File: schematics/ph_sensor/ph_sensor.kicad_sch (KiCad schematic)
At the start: 4 parts, among them U1 MCP3008

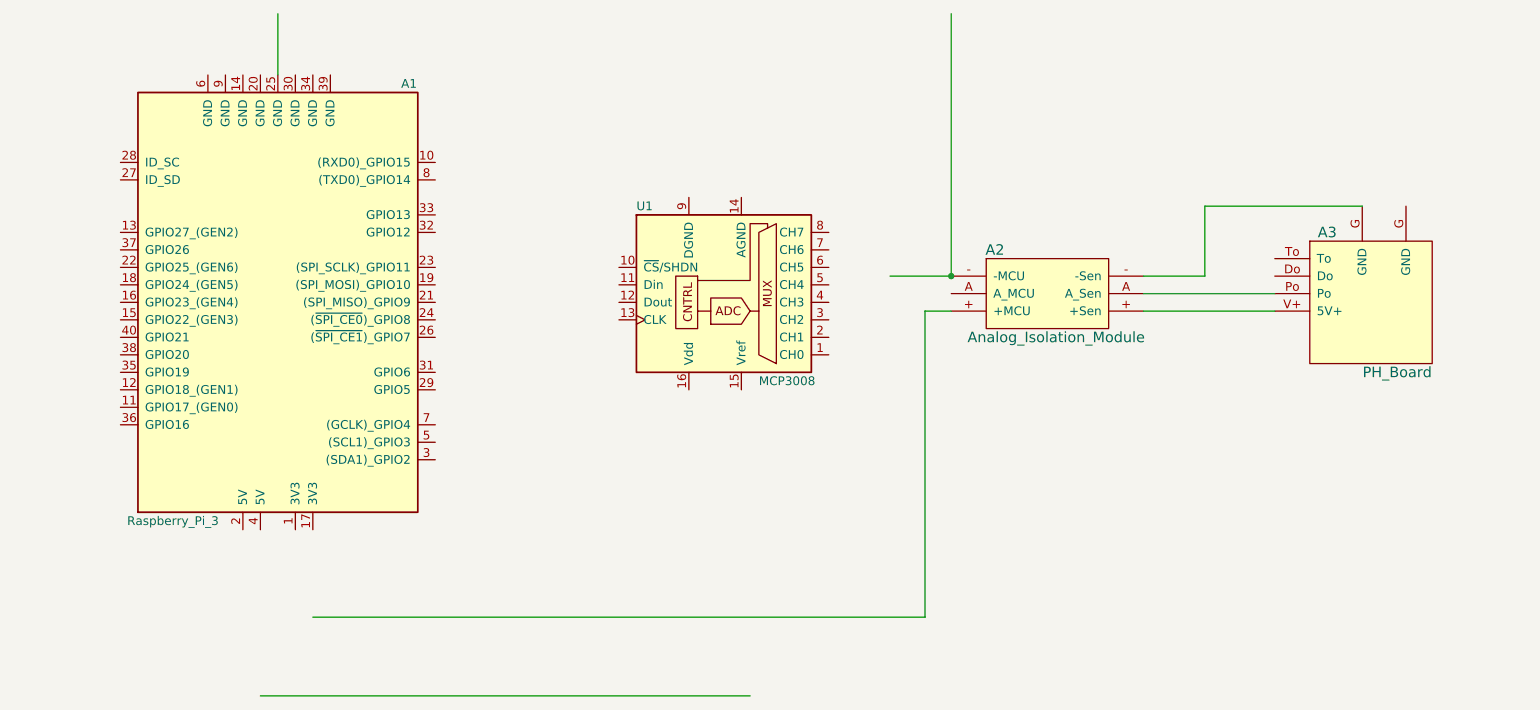
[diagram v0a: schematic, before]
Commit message: updated drawing
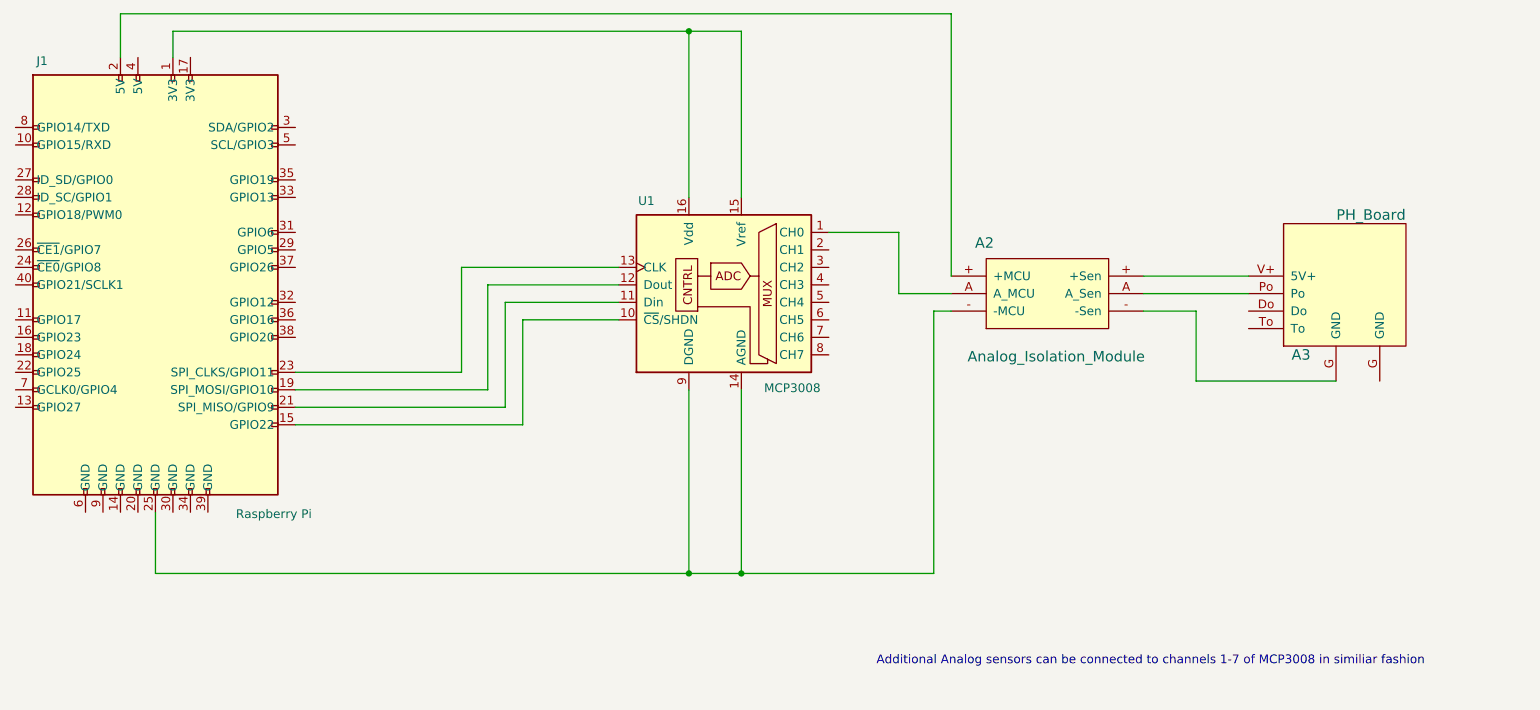
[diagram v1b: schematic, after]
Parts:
- removed A1: Raspberry_Pi_3, Pin_Headers:Pin_Header_Straight_2x20, symbol PH_Meter-rescue:Raspberry_Pi_2_3
- added J1: Raspberry Pi, symbol reefberrypi:Raspberry_Pi
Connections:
- net at A2.+ (+Sen): now also J1.2 (5V)
- net at A2.- (-Sen): now also U1.14 (AGND), U1.9 (DGND), J1.25 (GND)
- net at A3.G (GND): no longer A2.- (-Sen)
- net at A2.A (A_Sen): now also U1.1 (CH0)
- net at U1.10 (~{CS}/SHDN): now also J1.15 (GPIO22)
- net at U1.11 (Din): now also J1.21 (SPI_MISO/GPIO9)
- net at U1.12 (Dout): now also J1.19 (SPI_MOSI/GPIO10)
- net at U1.13 (CLK): now also J1.23 (SPI_CLKS/GPIO11)
- net at U1.15 (Vref): now also U1.16 (Vdd), J1.1 (3V3)
- new net: A2.- (-Sen), A3.G (GND)
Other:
- note added: "Additional Analog sensors can be connected to channels 1-7 of MCP3008 in similiar fashion"
- company: (none) -> ReefSpy Labs
- title: (none) -> Analog Sensors (PH)
- moved on the sheet: A3, U1
